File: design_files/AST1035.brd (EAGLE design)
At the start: 10 x 11 mm, 5 parts, among them J1 SM05B, J5 AST7525, Q1 2N7002P

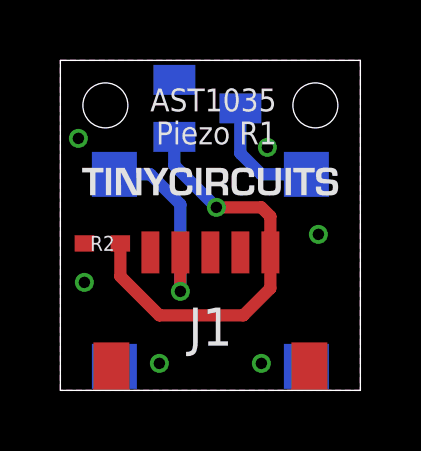
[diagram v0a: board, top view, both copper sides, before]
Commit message: update naming
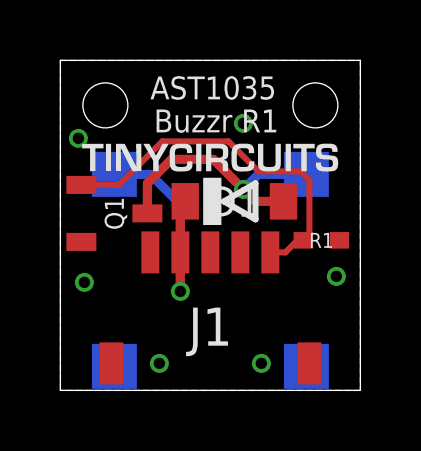
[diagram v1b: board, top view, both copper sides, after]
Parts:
- removed R2: 10.0K, tinycircuits:0402
- added D1: MBR120VLSFT1G, tinycircuits:SOD-123FL
- added R1: 10.0K, tinycircuits:0402
- J1: device tinycircuits:JST_SH_5X1 -> tinycircuits:JST_SH_5X1_EDGE
- Q1: device tinycircuits:SOT23 -> tinycircuits:SOT23A
- moved Q1 4.68 mm to (16.8, 15.9), flipped to the top, turned to 270 degrees
- renumbered J5 to J2
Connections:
- net GND: now also R1.1; no longer R2.1
- net INT: now also R1.2; no longer R2.2
- net LOAD: now also D1.A
- net VCC: now also D1.C
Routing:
- net LOAD: track 3.99 -> 8.76 mm, vias 0 -> 1
- net INT: track 14.3 -> 12.1 mm, vias 1 -> 0
- net VCC: track 6.81 -> 8.58 mm
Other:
- board text added: "Buzzr R1"
- board text added: "Wireling Buzzer"
- board text removed: "Piezo Board"
- board text removed: "Piezo R1"
